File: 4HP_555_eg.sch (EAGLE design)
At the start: 49 parts, among them IC1 IC_555-SOIC8, Q1 MMBT5088, Q2 MMBT5088, Q3 MMBT5088, Q4 MMBT5088

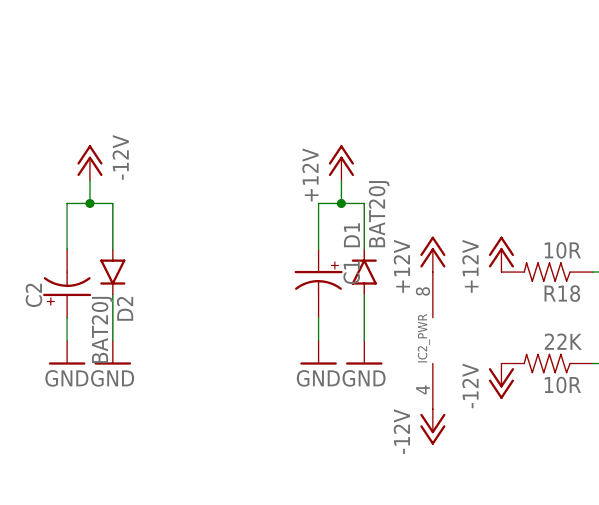
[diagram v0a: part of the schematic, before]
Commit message: 4HP 555 ADSR EG
LM555 ADSR Envelope Generator
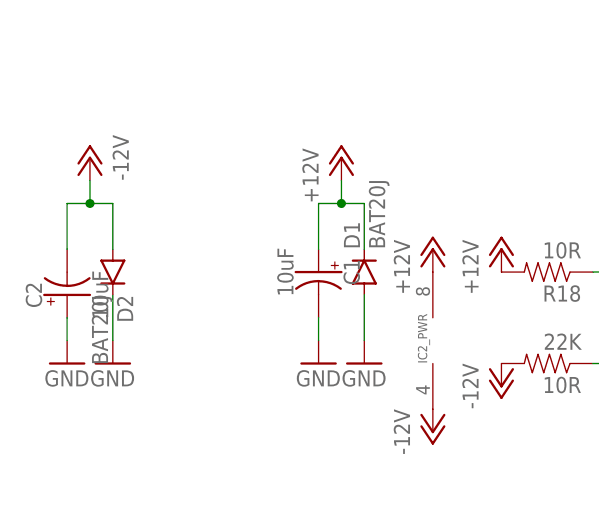
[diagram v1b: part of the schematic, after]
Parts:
- C1, C2: value (none) -> 10uF
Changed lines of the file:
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@@
 <?xml version="1.0" encoding="utf-8"?>
 <!DOCTYPE eagle SYSTEM "eagle.dtd">
-<eagle version="7.5.0">
+<eagle version="8.1.1">
 <drawing>
 <settings>
@@
 <part name="R11" library="SparkFun-Passives" deviceset="RESISTOR" device="0603-RES" value="1M"/>
 <part name="GND20" library="supply1" deviceset="GND" device=""/>
-<part name="C1" library="capacitors-elec" deviceset="050" device="1"/>
-<part name="C2" library="capacitors-elec" deviceset="050" device="1"/>
+<part name="C1" library="capacitors-elec" deviceset="050" device="1" value="10uF"/>
+<part name="C2" library="capacitors-elec" deviceset="050" device="1" value="10uF"/>
 <part name="R12" library="SparkFun-Passives" deviceset="RESISTOR" device="0603-RES" value="22K"/>
 <part name="R13" library="SparkFun-Passives" deviceset="RESISTOR" device="0603-RES" value="22K"/>
